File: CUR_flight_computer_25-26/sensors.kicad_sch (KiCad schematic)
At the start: 3 parts, among them U2 LPS22HB

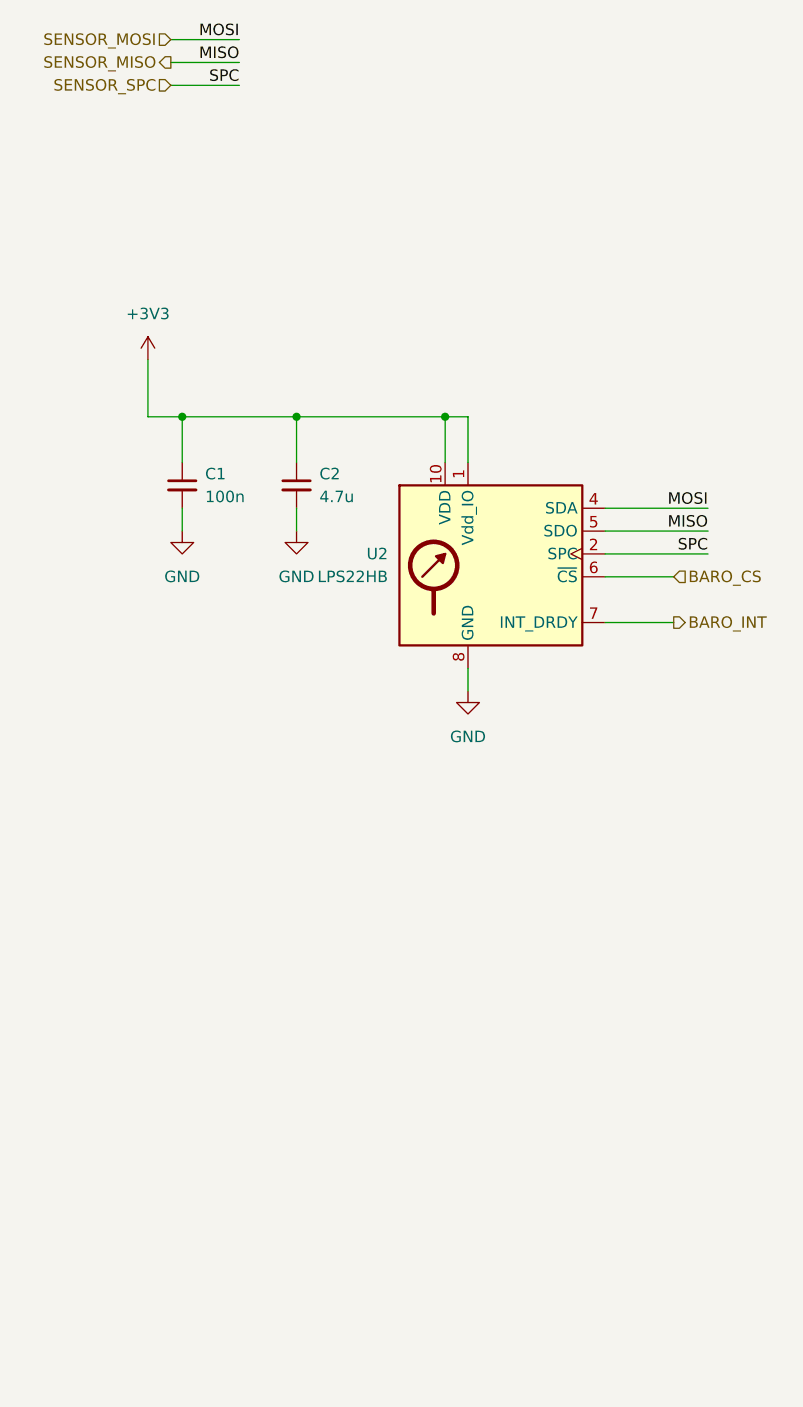
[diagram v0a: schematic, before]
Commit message: Magnitomer
Put In Magnitominer
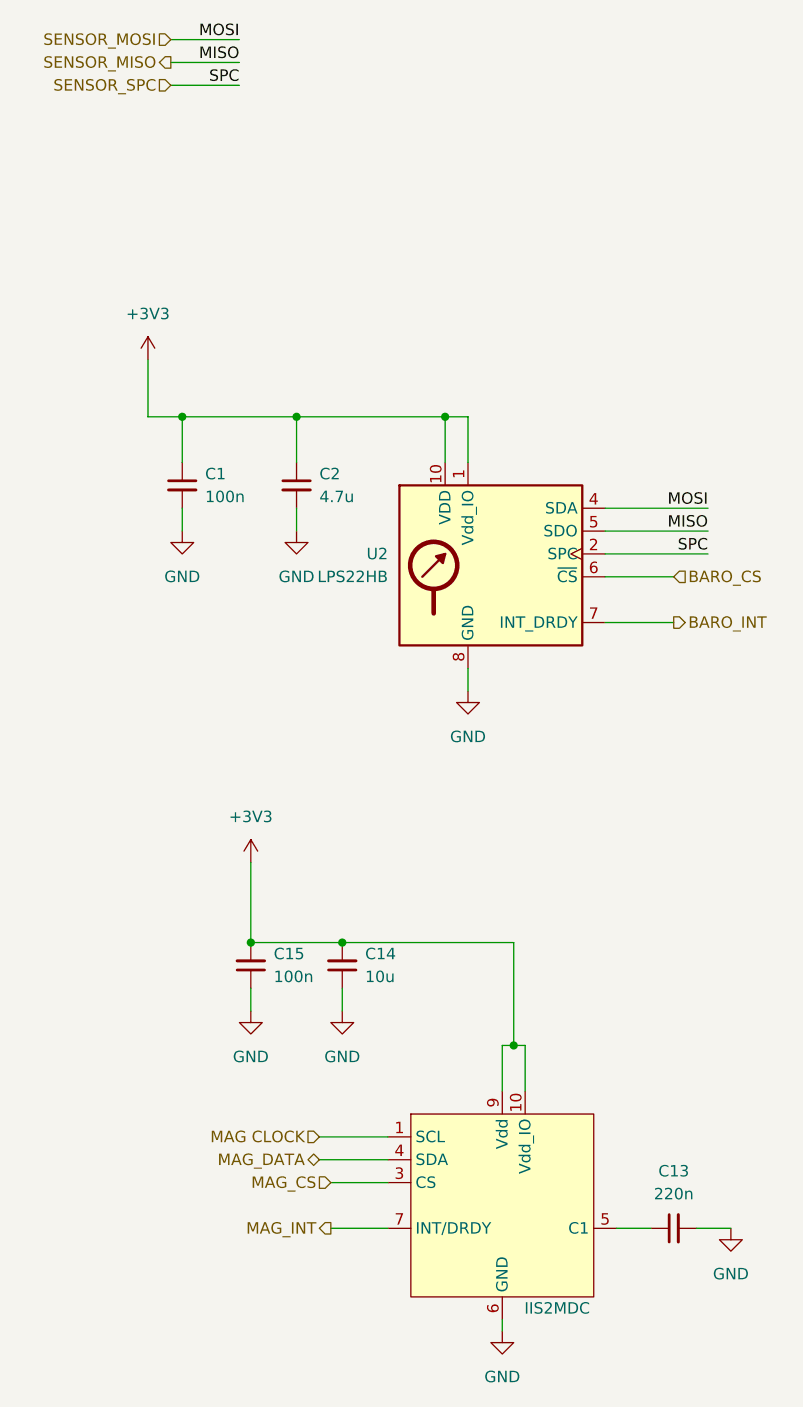
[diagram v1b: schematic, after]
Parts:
- added C13: 220n, symbol Device:C_Small
- added C14: 10u, symbol Device:C_Small
- added C15: 100n, symbol Device:C_Small
- added U1: IIS2MDC, ST_IIS2MDC:LGA-12_2X2X0P7_STM, symbol ST_Sensor_IMU:IIS2MDC
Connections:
- net +3V3: now also C14.2, C15.2, U1.10 (Vdd_IO), U1.9 (Vdd)
- net GND: now also C13.2, C14.1, C15.1, U1.6 (GND), U1.8 (GND)
- new net: U1.11 (NC), U1.12 (NC), U1.2 (NC)
- new net: C13.1, U1.5 (C1)
- new net MAG CLOCK: U1.1 (SCL)
- new net MAG_CS: U1.3 (CS)
- new net MAG_DATA: U1.4 (SDA)
- new net MAG_INT: U1.7 (INT/DRDY)
